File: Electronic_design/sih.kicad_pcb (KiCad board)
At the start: 2 copper layers, 20 parts, among them U1 ESP32-D0WD, U2 AP2112K-3.3, U3 TP4057, U4 LM358, Y1 40MHz

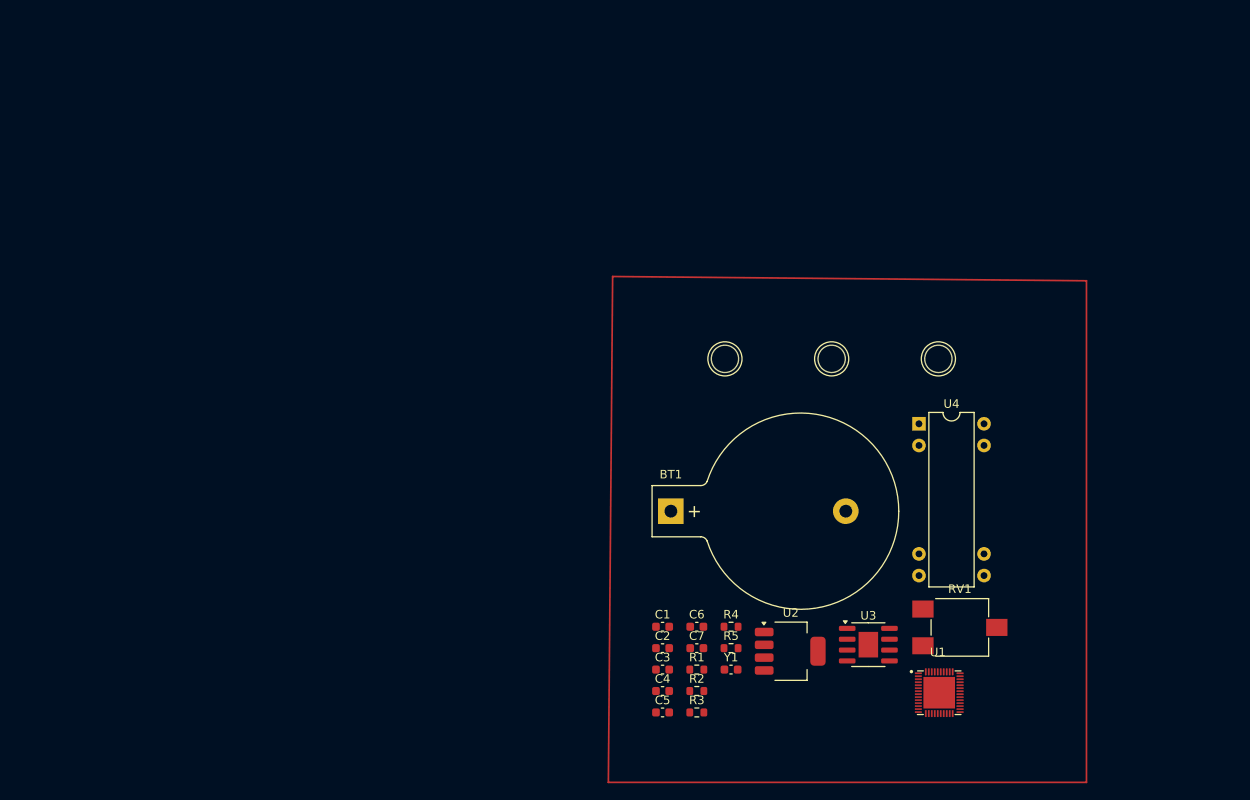
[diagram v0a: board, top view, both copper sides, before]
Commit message: PCB design and schematic modified
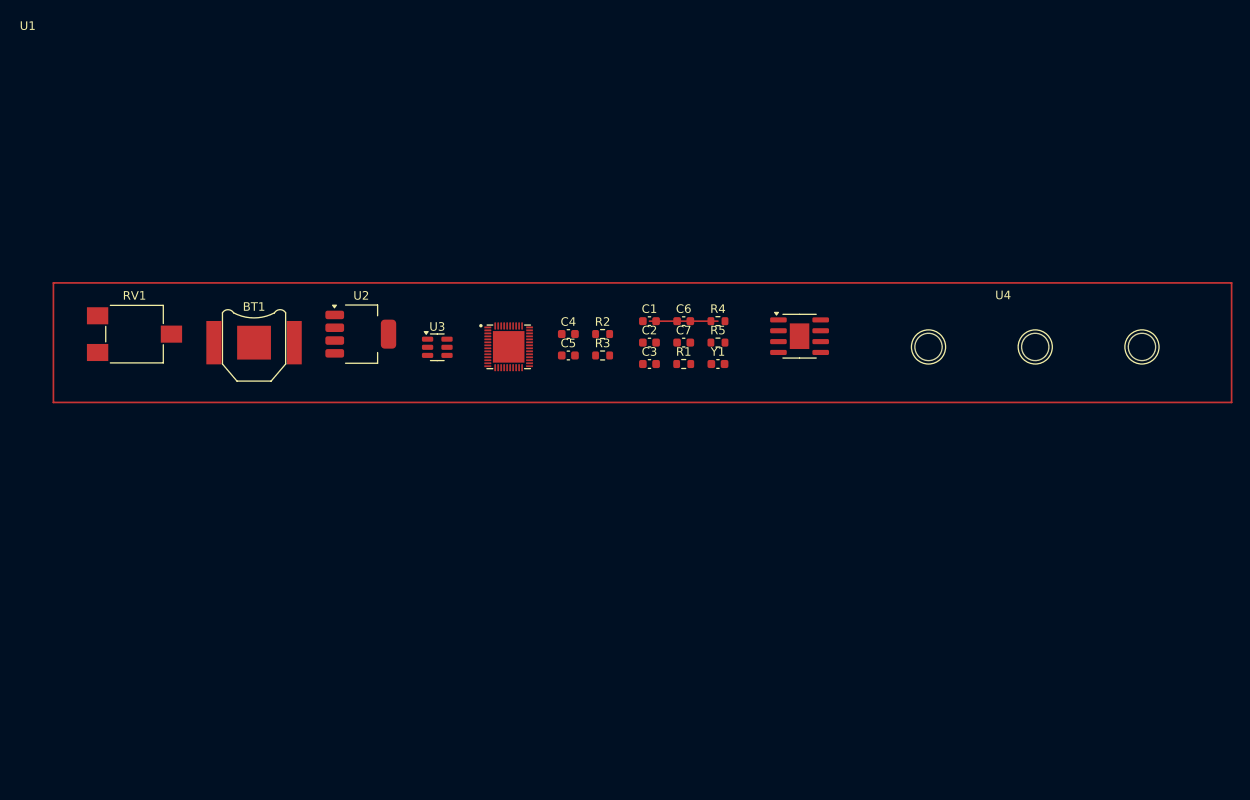
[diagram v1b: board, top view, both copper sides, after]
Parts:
- BT1: footprint Battery:BatteryHolder_Keystone_103_1x20mm -> Battery:BatteryHolder_Keystone_2998_1x6.8mm
- RV1: value R_Potentiometer -> 10 K
- U3: footprint Package_SO:SOIC-8-1EP_3.9x4.9mm_P1.27mm_EP2.29x3mm -> Package_TO_SOT_SMD:SOT-23-6
- U4: footprint Package_DIP:DIP-8-16_W7.62mm -> Package_SO:SOIC-8-1EP_3.9x4.9mm_P1.27mm_EP2.29x3mm
- moved RV1 102.6 mm to (57.5, 75.0)
- moved U1 64.7 mm to (101.3, 76.5)
- moved U2 62.5 mm to (84.0, 75.0)
- moved U3 61.3 mm to (93.0, 76.5)
- moved BT1 52.7 mm to (71.5, 76.0)
- moved C4 43.2 mm to (108.3, 75.0)
- moved C5 43.2 mm to (108.3, 77.5)
- moved R2 43.2 mm to (112.3, 75.0)
- moved R3 43.2 mm to (112.3, 77.5)
- moved C2 35.8 mm to (117.8, 76.0)
- moved C3 35.8 mm to (117.8, 78.5)
- moved C7 35.8 mm to (121.8, 76.0)
- moved R1 35.8 mm to (121.8, 78.5)
- moved R5 35.8 mm to (125.8, 76.0)
- moved Y1 35.8 mm to (125.8, 78.5)
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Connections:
- C7 pad 2: GND -> Net-(U4A-+)
- R2 pad 2: 3.3V -> Net-(U2-VOUT)
- R3 pad 1: 3.3V -> Net-(U2-VOUT)
- R3 pad 2: GND -> Net-(U4A-+)
- R4 pad 2: GND -> Net-(U4A-+)
- RV1 pad 2: GND -> Net-(U4A-+)
- U4 pad 3: GND -> Net-(U4A-+)
